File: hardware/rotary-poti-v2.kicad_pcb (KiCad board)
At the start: 2 copper layers, 30 x 25 mm, 22 parts, among them P1 CON-SENSOR2, P2 DEBUG, P3 BOOT, U1 XMC1XXX24, U3 DRILL, U4 DRILL, U5 DRILL, U6 DRILL

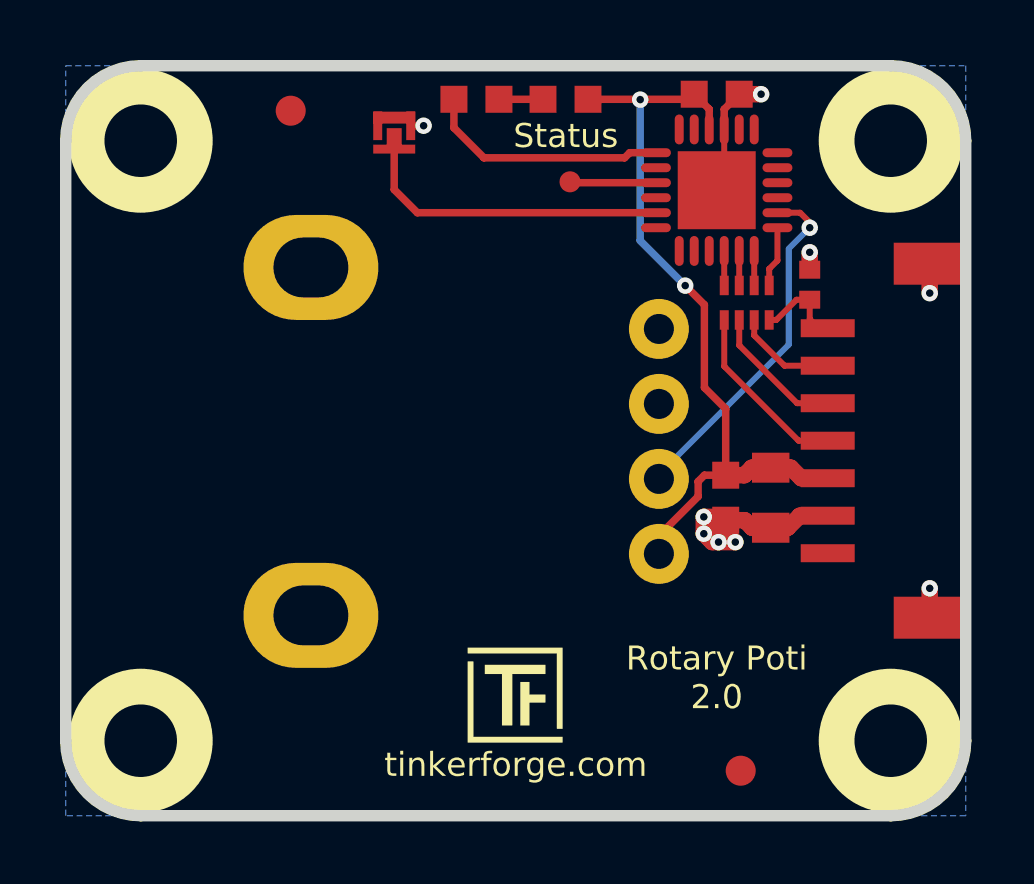
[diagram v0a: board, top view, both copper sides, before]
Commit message: Fix origin
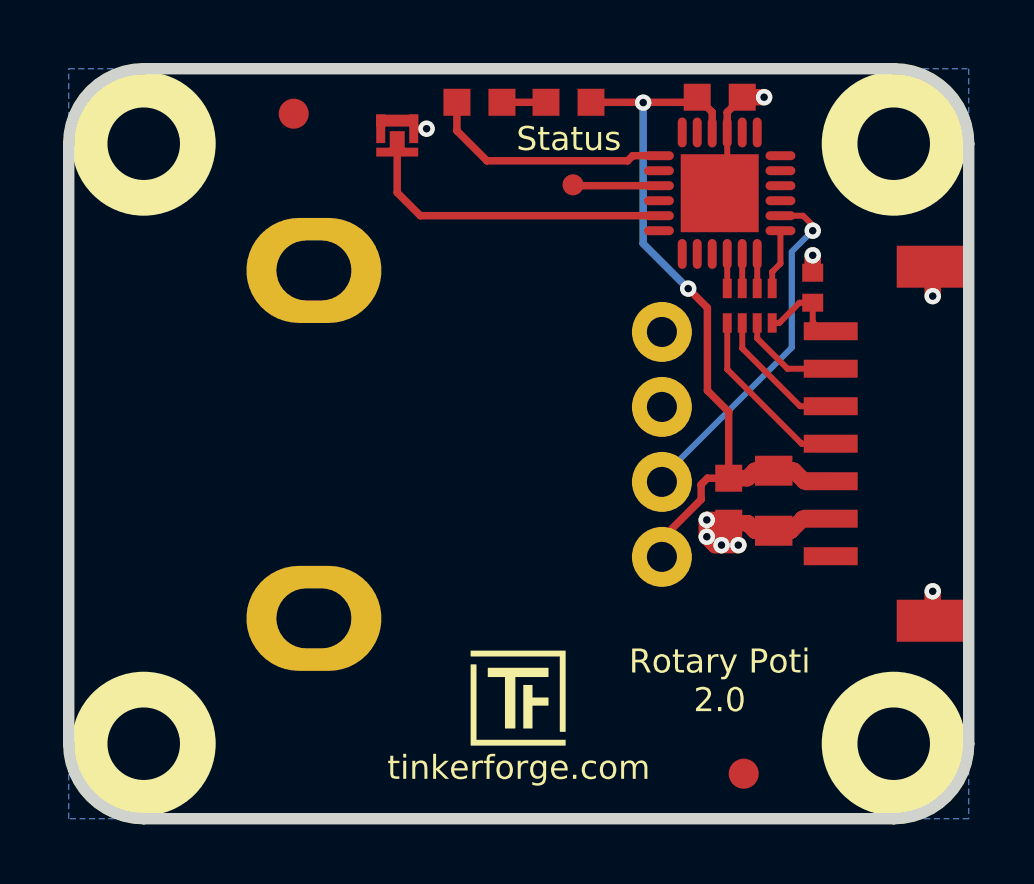
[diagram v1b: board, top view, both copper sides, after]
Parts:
- moved VAL 0.14 mm to (157.3, 102.2)
- moved VAL 0.14 mm to (149.3, 102.2)
- moved Ref** 0.14 mm to (146.8, 109.1)
- moved C5 0.14 mm to (155.1, 90.7)
- moved Fiducial_Mark 0.14 mm to (155.9, 113.2)
- moved Fiducial_Mark 0.14 mm to (140.9, 91.2)
- moved G*** 0.14 mm to (141.9, 102.2)
- moved P1 0.14 mm to (163.4, 102.2)
- moved P3 0.14 mm to (144.3, 91.9)
- moved RV1 0.14 mm to (147.7, 102.2)
- moved U3 0.14 mm to (135.9, 112.2)
- moved U4 0.14 mm to (160.9, 92.2)
- moved U5 0.14 mm to (160.9, 112.2)
- moved U6 0.14 mm to (135.9, 92.2)
- moved C1 0.14 mm to (158.2, 97.0)
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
